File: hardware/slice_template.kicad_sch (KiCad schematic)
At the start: 24 parts, among them J1 Conn_01x10_Socket, SW1 SW_DIP_x04, U1 AP63205, U2 PCA9306DC1

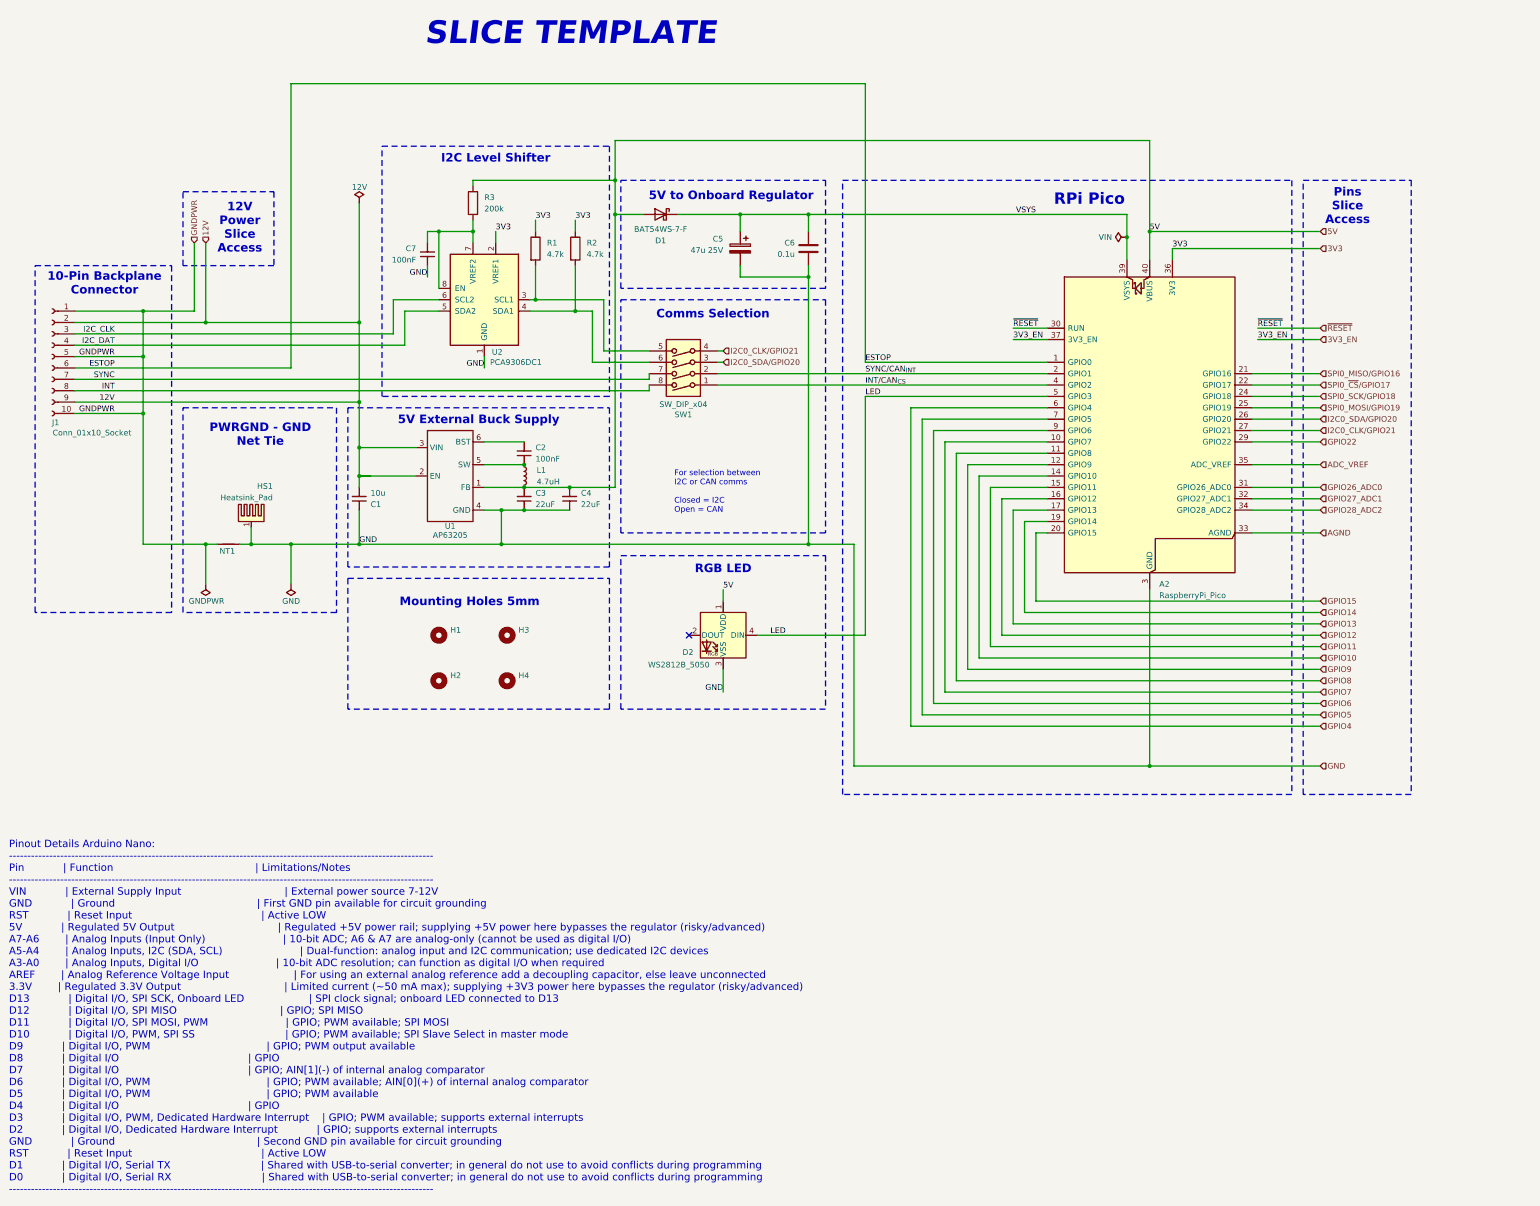
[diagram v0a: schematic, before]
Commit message: finished layout
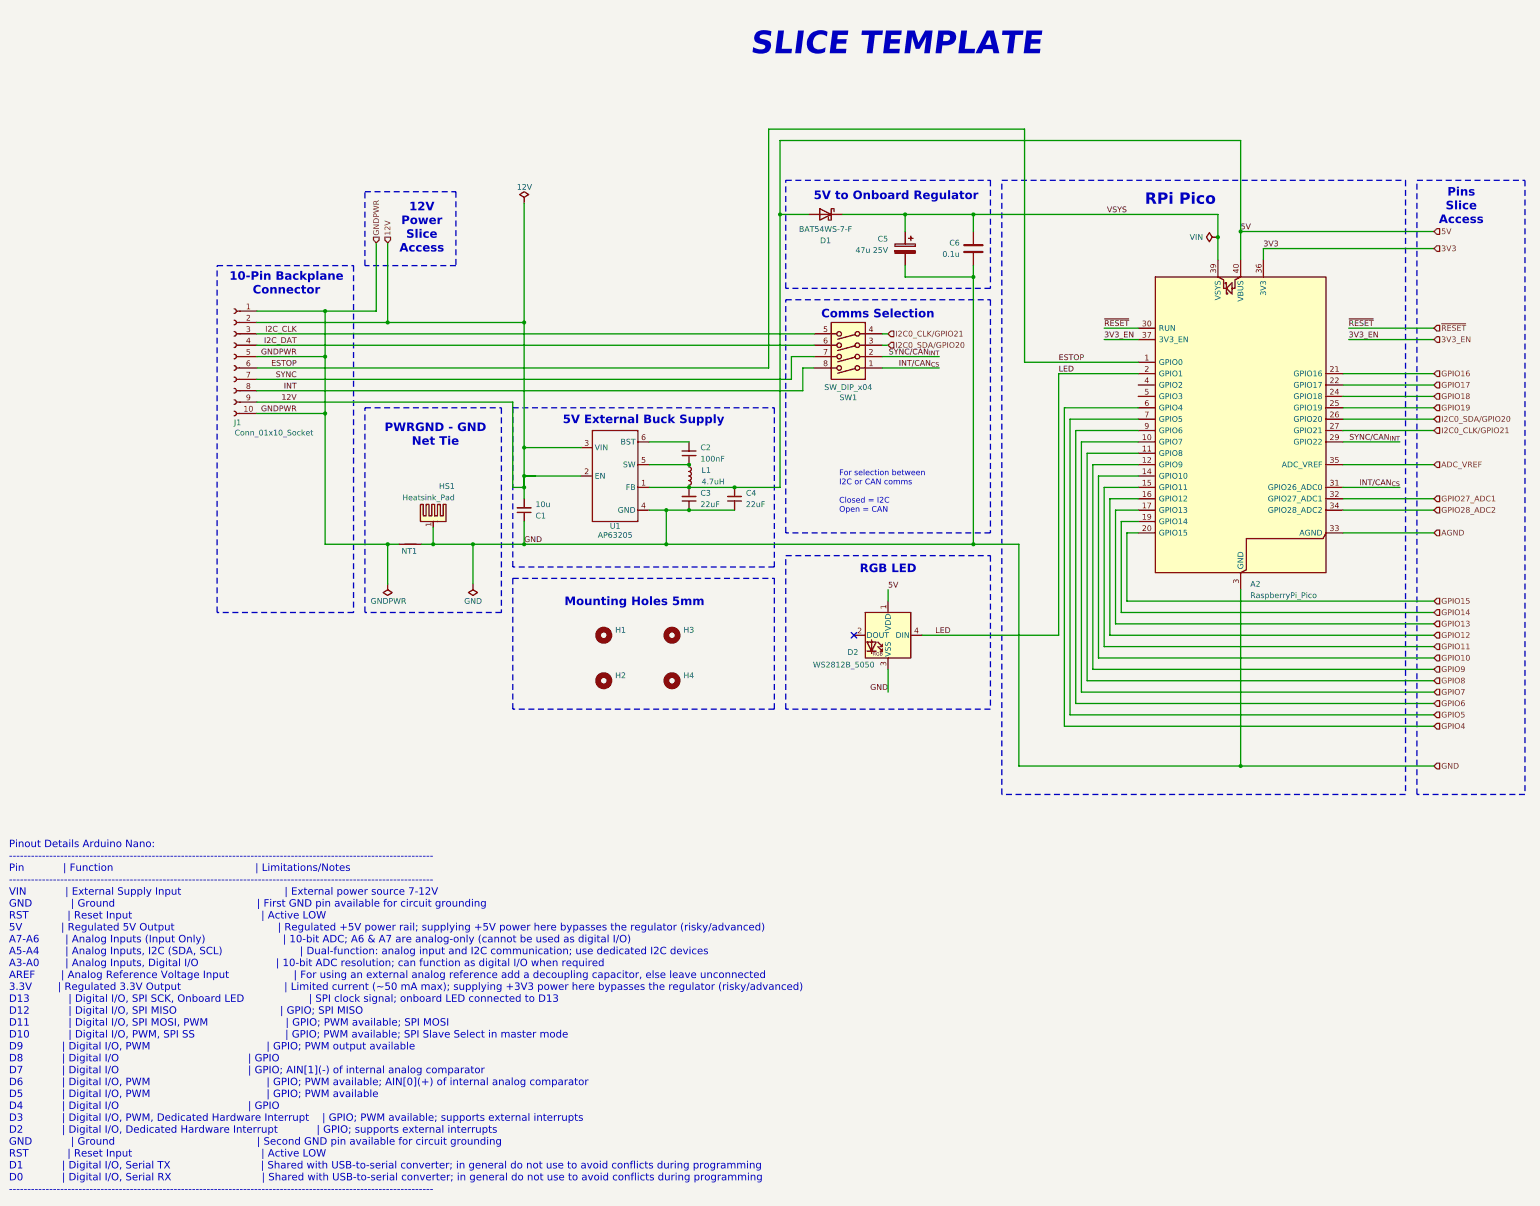
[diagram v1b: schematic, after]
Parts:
- removed C7: 100nF, Capacitor_SMD:C_1206_3216Metric, symbol Device:C_Small
- removed R1, R2: 4.7k, Resistor_SMD:R_0603_1608Metric_Pad0.98x0.95mm_HandSolder, symbol Device:R
- removed R3: 200k, Resistor_SMD:R_0603_1608Metric_Pad0.98x0.95mm_HandSolder, symbol Device:R
- removed U2: PCA9306DC1, Package_SO:VSSOP-8_2.3x2mm_P0.5mm, symbol Interface:PCA9306DC1
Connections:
- net GPIO22 is gone; now on net SYNC/CAN_{INT}: A2.29 (GPIO22)
- net GPIO26_ADC0 is gone; now on net INT/CAN_{CS}: A2.31 (GPIO26_ADC0)
- net I2C_CLK: now also SW1.5
- net I2C_DAT: now also SW1.6
- net INT/CAN_{CS}: no longer A2.4 (GPIO2)
- net LED: now also A2.2 (GPIO1); no longer A2.5 (GPIO3)
- net SYNC/CAN_{INT}: no longer A2.2 (GPIO1)
- net SPI0_MISO/GPIO16 renamed GPIO16
- net SPI0_MOSI/GPIO19 renamed GPIO19
- net SPI0_SCK/GPIO18 renamed GPIO18
- net SPI0_~{CS}/GPIO17 renamed GPIO17
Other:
- note removed: "I2C Level Shifter"
- moved on the sheet: A2, C1, C2, C3, C4, C5, C6, D1, D2, H1, H2, H3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
